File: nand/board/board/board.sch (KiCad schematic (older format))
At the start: 40 parts, among them J1 Conn_01x13, J2 SWD1, J3 gnd, J4 SWD3, J5 3v3, J6 SWD2, J7 Raspberry_Pi_2_3, SW1 PTS645SJH73LFS, SW2 PTS645SJH73LFS, SW3 PTS645SJH73LFS, U1 STM32F303RDTx, U2 STM32F303RDTx, U3 STM32F303RDTx, Y1 8 MHz, Y2 8 MHz, Y3 8 MHz

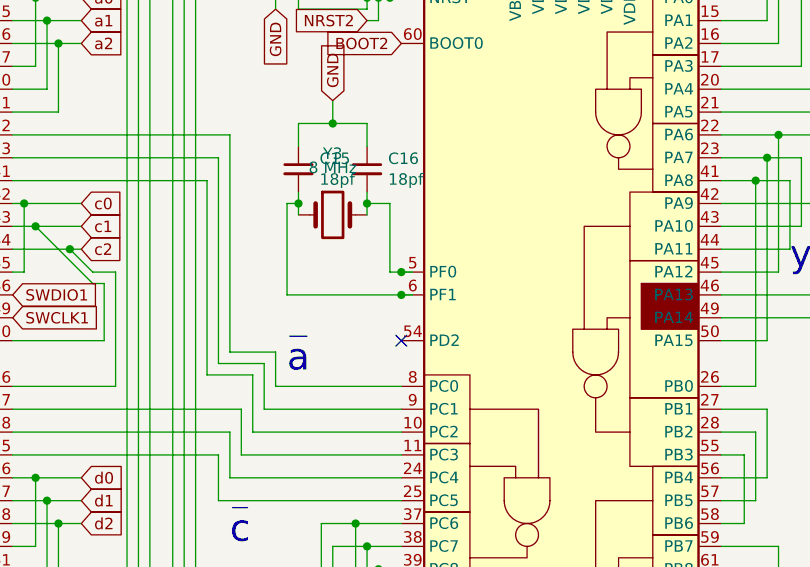
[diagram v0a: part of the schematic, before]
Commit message: v1 board sent for manufacturing
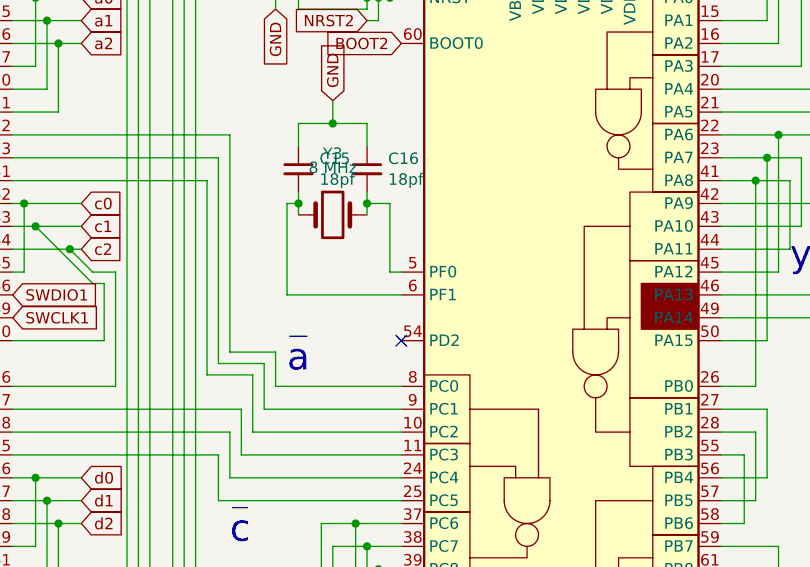
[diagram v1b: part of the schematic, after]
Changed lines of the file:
@@
 EESchema Schematic File Version 4
+LIBS:board-cache
 EELAYER 26 0
 EELAYER END
@@
 Wire Wire Line
 	4150 2250 4300 2250
-Connection ~ 4450 2900
-Wire Wire Line
-	4450 2900 4500 2900
-Connection ~ 4450 3000
-Wire Wire Line
-	4450 3000 4500 3000
 $Comp
 L boardparts:PTS645SJH73LFS SW1
